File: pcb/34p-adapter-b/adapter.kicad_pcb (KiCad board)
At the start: 2 copper layers, 30 x 21 mm, 9 parts, among them J1 FH12-40S-0.5SH, J2 FH34S-34S-0.5SH(50)

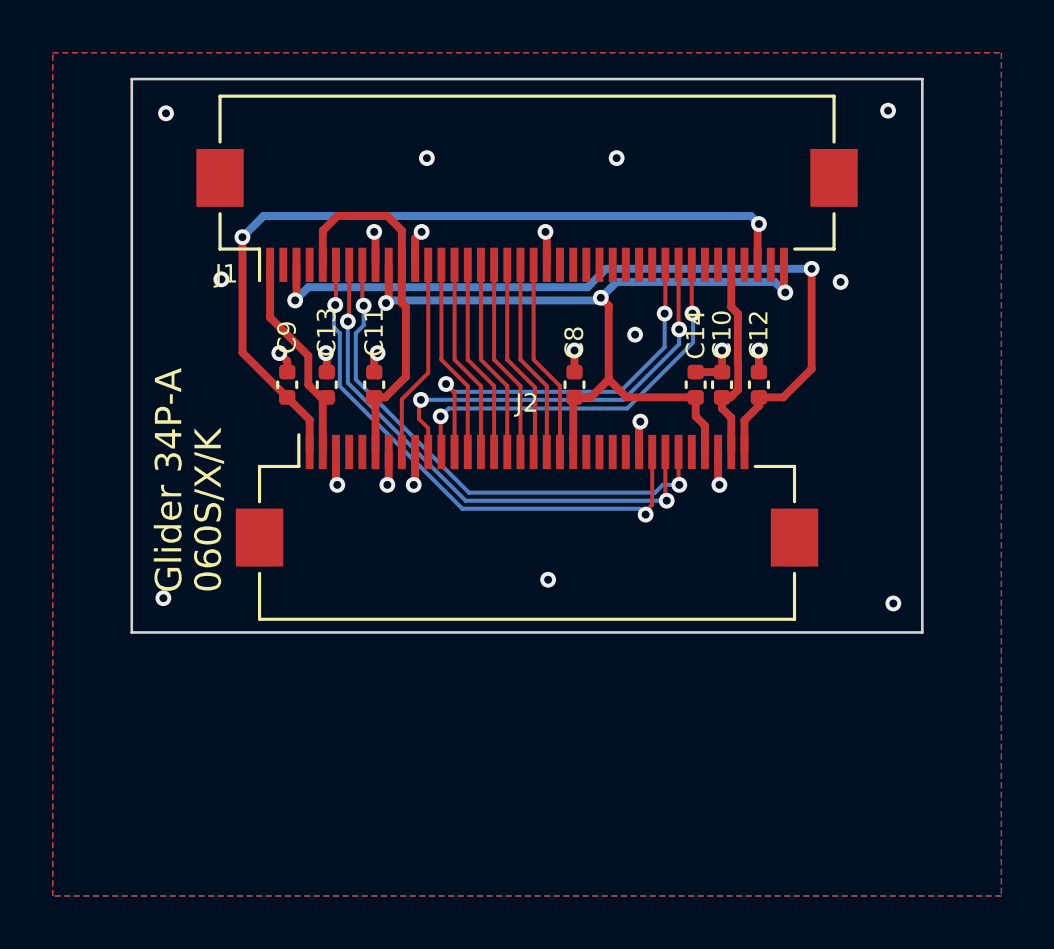
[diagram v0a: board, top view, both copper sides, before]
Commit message: Update adapters
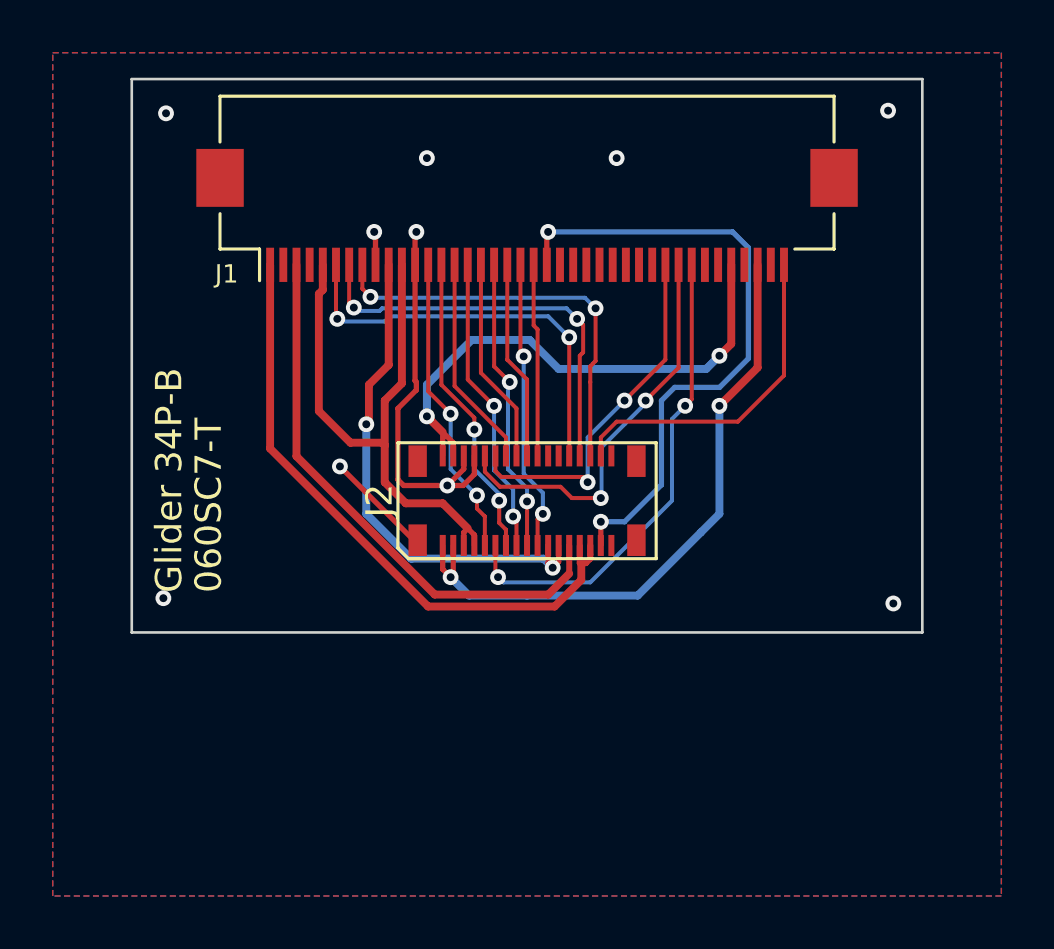
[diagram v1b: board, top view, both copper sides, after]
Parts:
- removed C10, C11, C12, C13, C14, C8, C9: 220nF, Capacitor_SMD:C_0402_1005Metric
- J2: value FH34S-34S-0.5SH(50) -> AXT334124; footprint Connector_FFC-FPC:Hirose_FH12-34S-0.5SH_1x34-1MP_P0.50mm_Horizontal -> footprints:AXT334124
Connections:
- J1 pad 40: VCOM -> /BORDER
- J2 pad 2: VGL -> VPOS
- J2 pad 23: unconnected-(J2-Pad23) -> VCOM
- J2 pad 25: unconnected-(J2-Pad25) -> VGH
- J2 pad 26: GND -> /GDOE
- J2 pad 27: /GDOE -> VGL
- J2 pad 29: /GDSP -> VGL
- J2 pad 3: GND -> VNEG
- J2 pad 30: unconnected-(J2-Pad30) -> /GDSP
- J2 pad 31: VCOM -> GND
- J2 pad 32: GND -> /BORDER
- J2 pad 33: VPOS -> unconnected-(J2-Pin_33-Pad33)
- J2 pad 34: VGH -> unconnected-(J2-Pin_34-Pad34)
- J2 pad 4: unconnected-(J2-Pad4) -> VPOS
- J2 pad 5: unconnected-(J2-Pad5) -> +3V3
- J2 pad 6: +3V3 -> GND
- J2 pad 7: GND -> +3V3
- J2 pad 8: /ESDCLK -> GND
- J2 pad 9: GND -> /ESDCLK
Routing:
- net GND: track 16.0 -> 44.6 mm, vias 24 -> 12
- net VGL: track 8.18 -> 24.0 mm
- net /BORDER: track 0.00 -> 12.8 mm
- net VPOS: track 7.79 -> 20.1 mm, vias 0 -> 2
- net VCOM: track 30.9 -> 19.6 mm, vias 3 -> 2
- net VGH: track 30.0 -> 21.2 mm, vias 2 -> 0
- net +3V3: track 14.0 -> 22.5 mm
- net VNEG: track 30.8 -> 24.4 mm
- net /GDOE: track 20.8 -> 15.8 mm
- net /GDCLK: track 20.3 -> 15.8 mm
- net /GDSP: track 19.9 -> 15.7 mm
- net /ED0: track 7.51 -> 11.7 mm, vias 0 -> 2
- net /ESDCLK: track 7.51 -> 11.5 mm, vias 0 -> 2
- net /ED2: track 7.51 -> 11.4 mm, vias 0 -> 2
- net /ED4: track 7.51 -> 11.2 mm, vias 0 -> 2
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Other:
- board text added: "060SC7-T"
- board text added: "Glider 34P-B"
- board text removed: "060S/X/K"
- board text removed: "Glider 34P-A"
